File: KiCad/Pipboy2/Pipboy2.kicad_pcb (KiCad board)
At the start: 2 copper layers, 61.4 x 57.4 mm, 20 parts

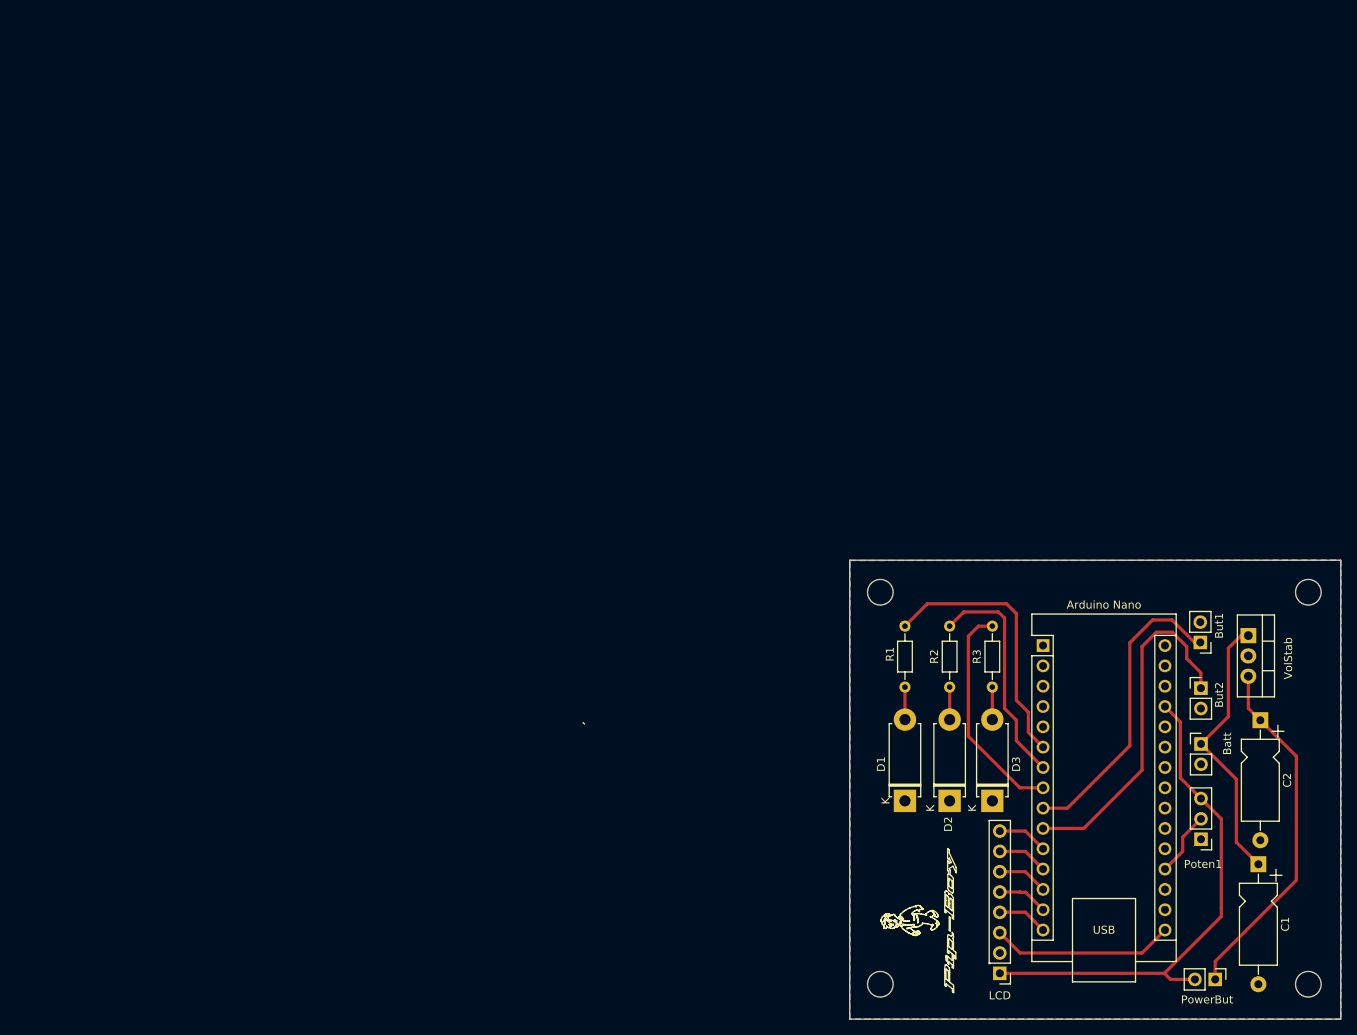
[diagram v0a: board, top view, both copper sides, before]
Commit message: Exported steps
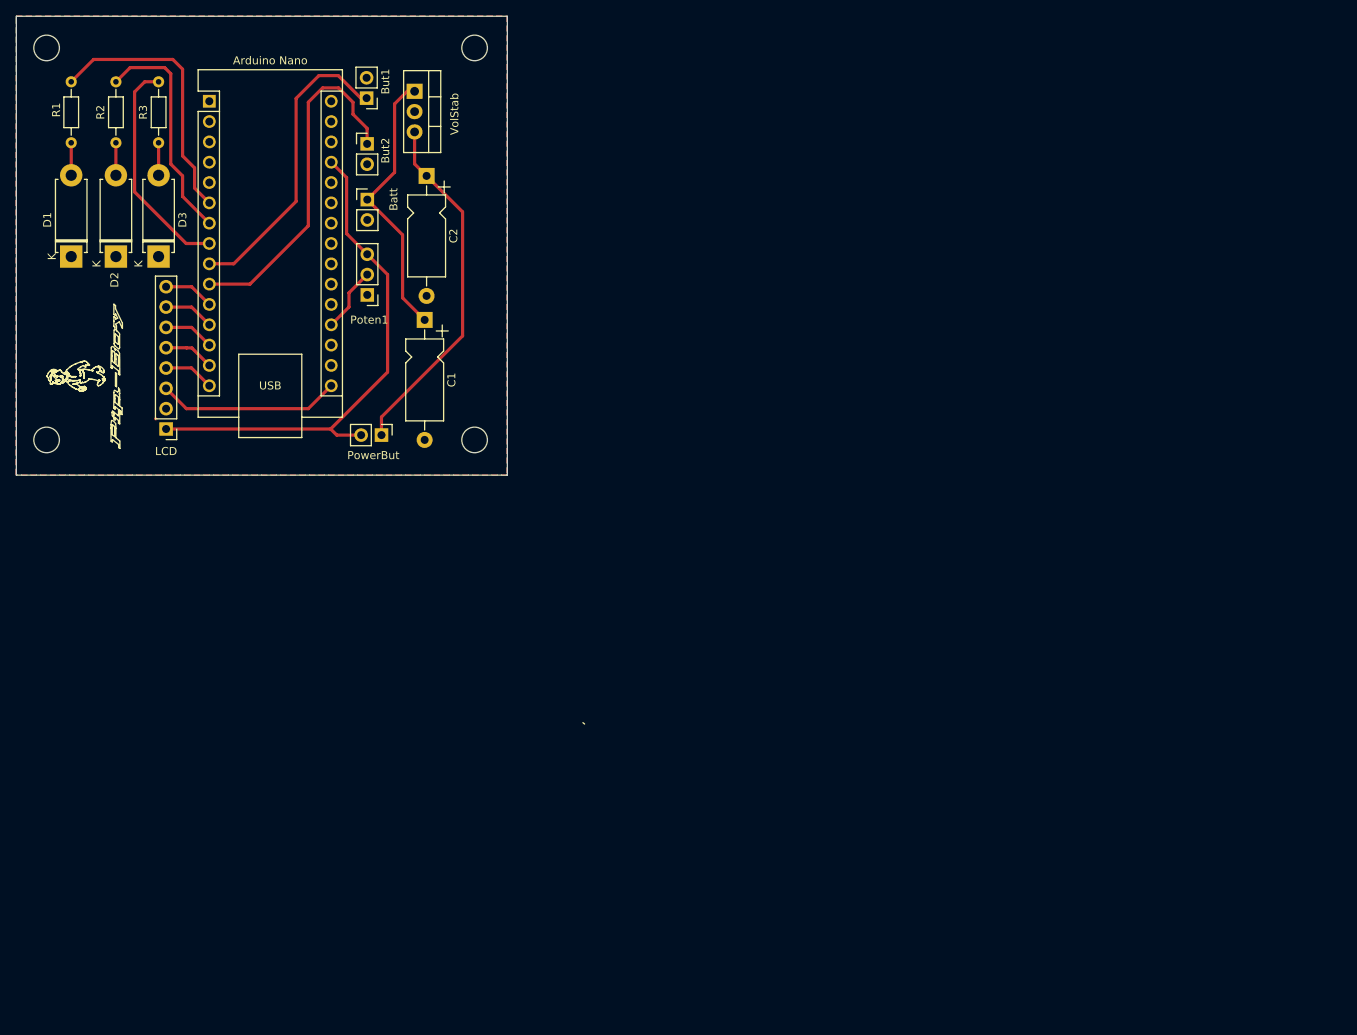
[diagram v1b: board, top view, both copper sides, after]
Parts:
- moved Arduino Nano 124.5 mm to (24.1, 10.6)
- moved Batt 124.5 mm to (43.9, 22.9)
- moved But1 124.5 mm to (43.8, 10.2)
- moved But2 124.5 mm to (43.9, 16.0)
- moved C2 124.5 mm to (51.3, 20.0)
- moved D1 124.5 mm to (6.86, 30.0)
- moved D2 124.5 mm to (12.4, 30.0)
- moved D3 124.5 mm to (17.8, 30.0)
- moved H1 124.5 mm to (57.3, 3.96)
- moved H2 124.5 mm to (3.78, 3.96)
- moved H3 124.5 mm to (3.78, 53.0)
- moved H4 124.5 mm to (57.3, 53.0)
- moved LCD 124.5 mm to (18.7, 51.6)
- moved PowerBut 124.5 mm to (45.6, 52.4)
- moved R1 124.5 mm to (6.86, 15.8)
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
